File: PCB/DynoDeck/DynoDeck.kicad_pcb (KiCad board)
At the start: 4 copper layers, 105 x 107.3 mm, 76 parts, among them J1 USB_C_Receptacle_USB2.0_16P, J2 PGRM, J3 CardKBConn, J4 E-paper, J5 HC-IPEX0125-01 (u.FL), J6 BWSMA-KWE-Z001 (SMA), J7 CardKBRef, SW1 QON, SW2 POWER, SW3 RESET, SW4 IO1, U1 BQ25895RTW, U2 USBLC6-2SC6, U3 SX1262IMLTRT, U4 TUSB320, U5 MD7218E33PC1, U6 E73-2G4M08S1C, U7 PE42422MLAA-Z, U8 PE42422MLAA-Z, Y1 OW7EL89CENUXK7YLC-32M, Y3 3N00032G33YC

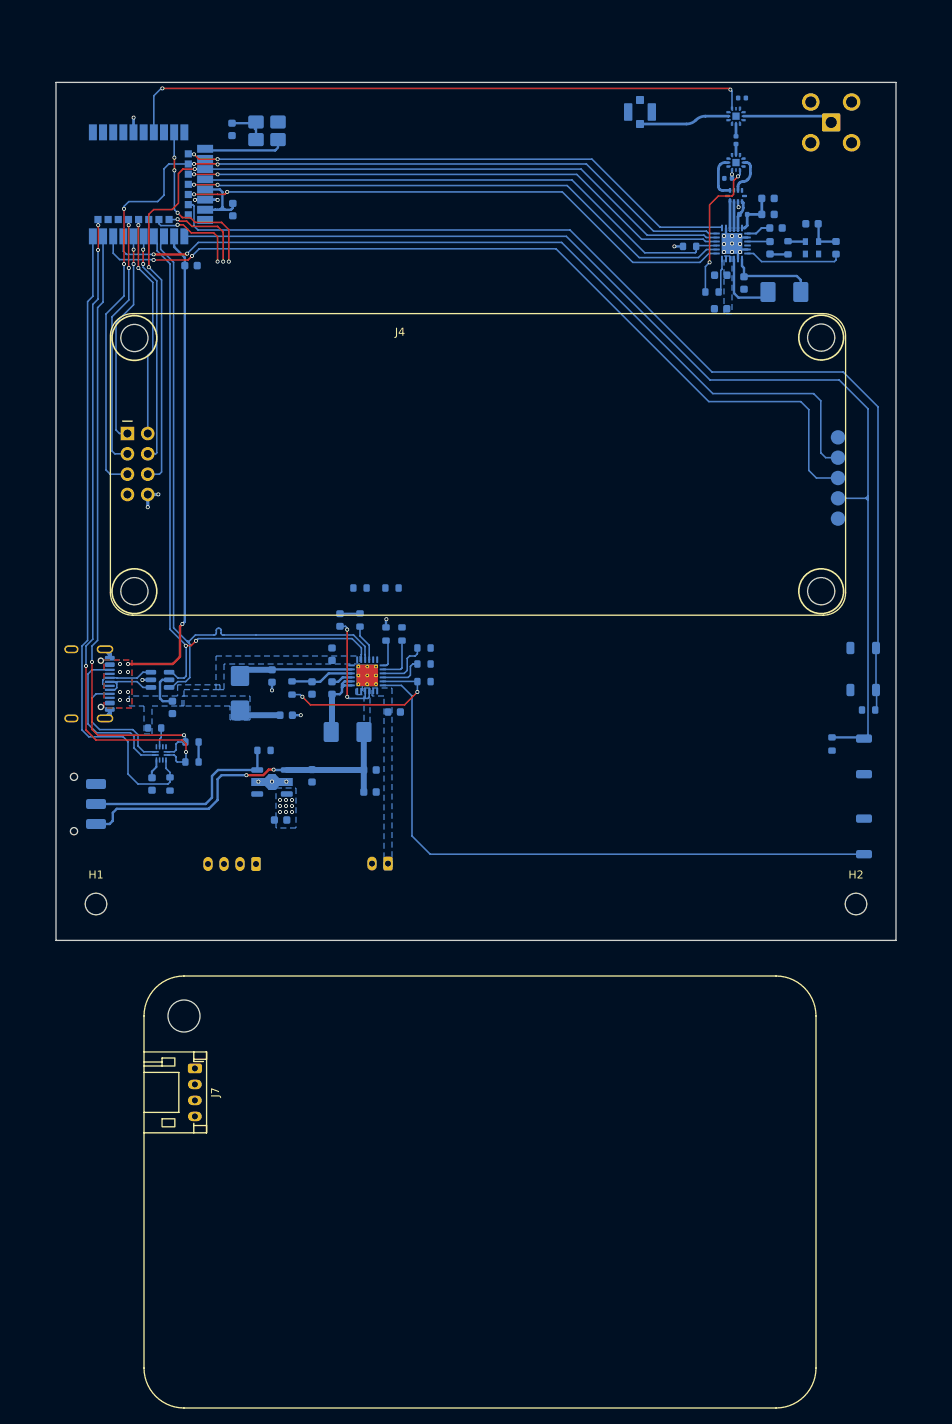
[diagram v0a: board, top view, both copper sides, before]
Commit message: nRF wiring finish I think
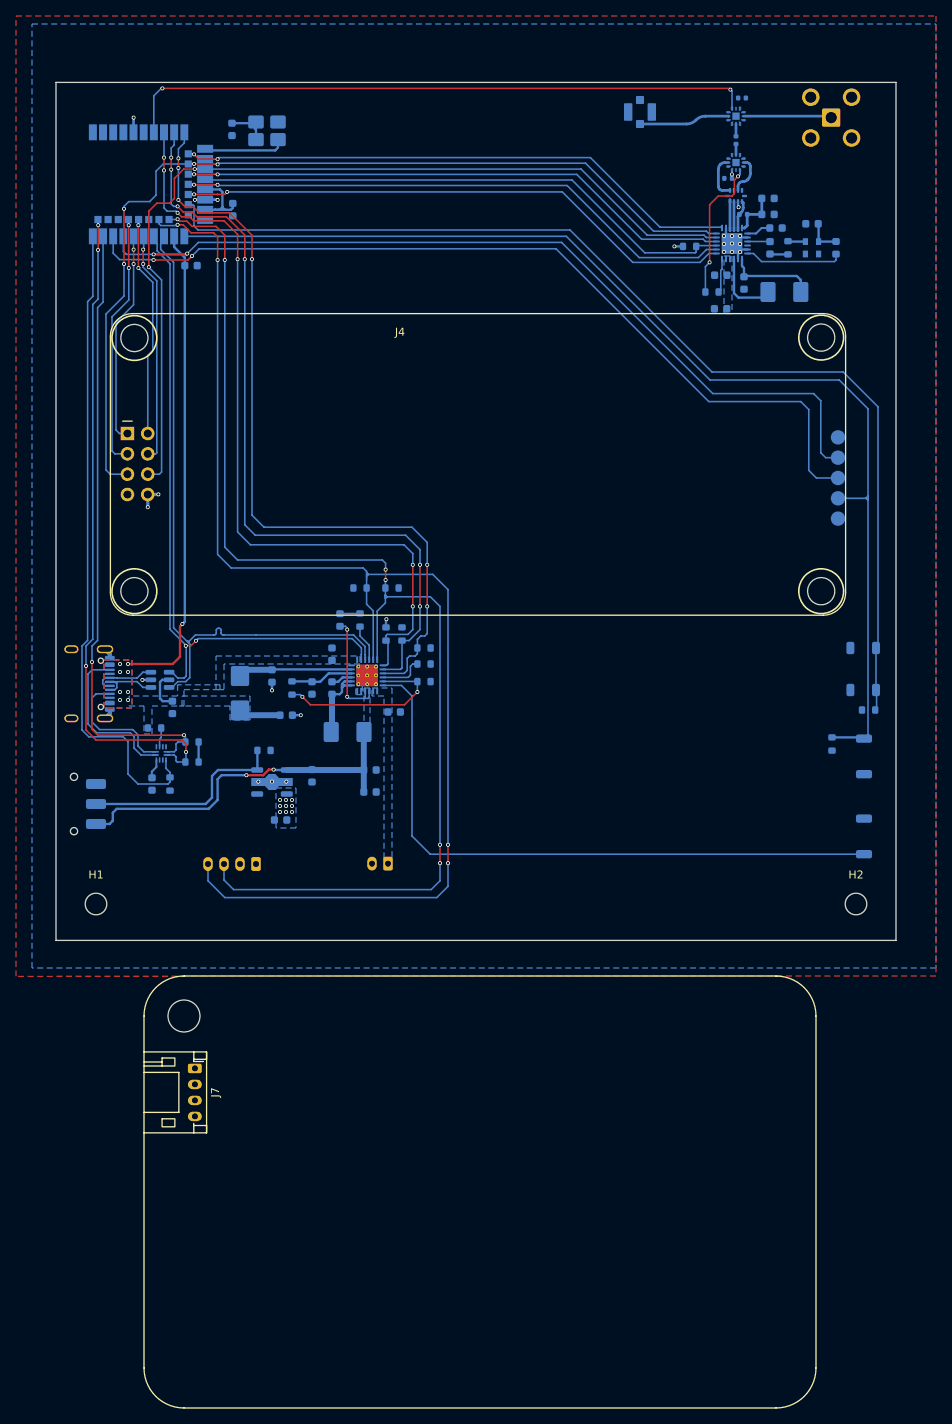
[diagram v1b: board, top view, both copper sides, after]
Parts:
- moved J6 0.60 mm to (126.9, 32.7)
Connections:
- U6 pad 10: /OTG -> /~{CE}
- U6 pad 28: unconnected-(U6B-P0.15-Pad28) -> /SDA
- U6 pad 30: unconnected-(U6B-P0.17-Pad30) -> /SCL
- U6 pad 9: /~{CE} -> /OTG
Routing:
- net /SCL: track 0.00 -> 161.5 mm, vias 0 -> 4
- net /SDA: track 0.00 -> 152.4 mm, vias 0 -> 6
- net /~{INT}: track 3.74 -> 97.8 mm, vias 0 -> 6
- net /OTG: track 5.46 -> 97.6 mm, vias 0 -> 6
- net /~{CE}: track 28.4 -> 99.0 mm, vias 4 -> 6
- net unconnected-(U6B-P0.17-Pad30): track 11.7 -> 0.00 mm, vias 2 -> 0
- net unconnected-(U6B-P0.15-Pad28): track 11.1 -> 0.00 mm, vias 2 -> 0
- added copper zone on F.Cu, net GND
